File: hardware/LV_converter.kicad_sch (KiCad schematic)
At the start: 29 parts, among them IC3 AP74502QTA8-7, J9 Conn_01x02, Q11 IRLML0030, Q4 NVMFWS1D7N04XMT1G, Q5 NVMFWS1D7N04XMT1G, U8 INA228

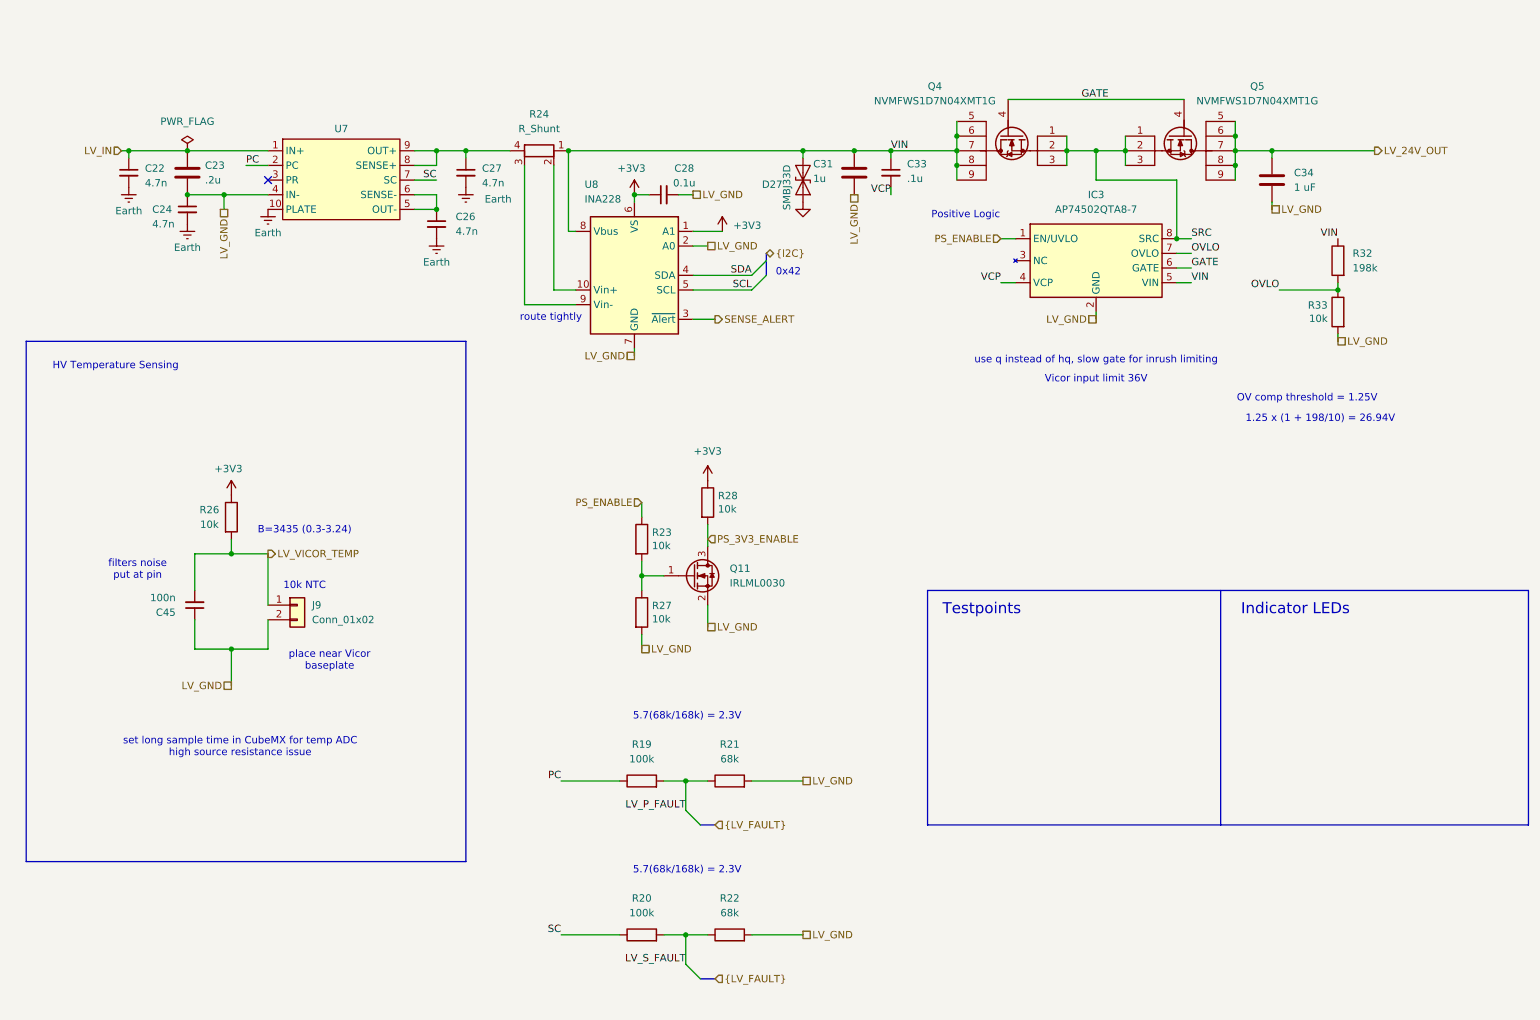
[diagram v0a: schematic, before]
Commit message: more fix, clean up, add some debug led and testpoints
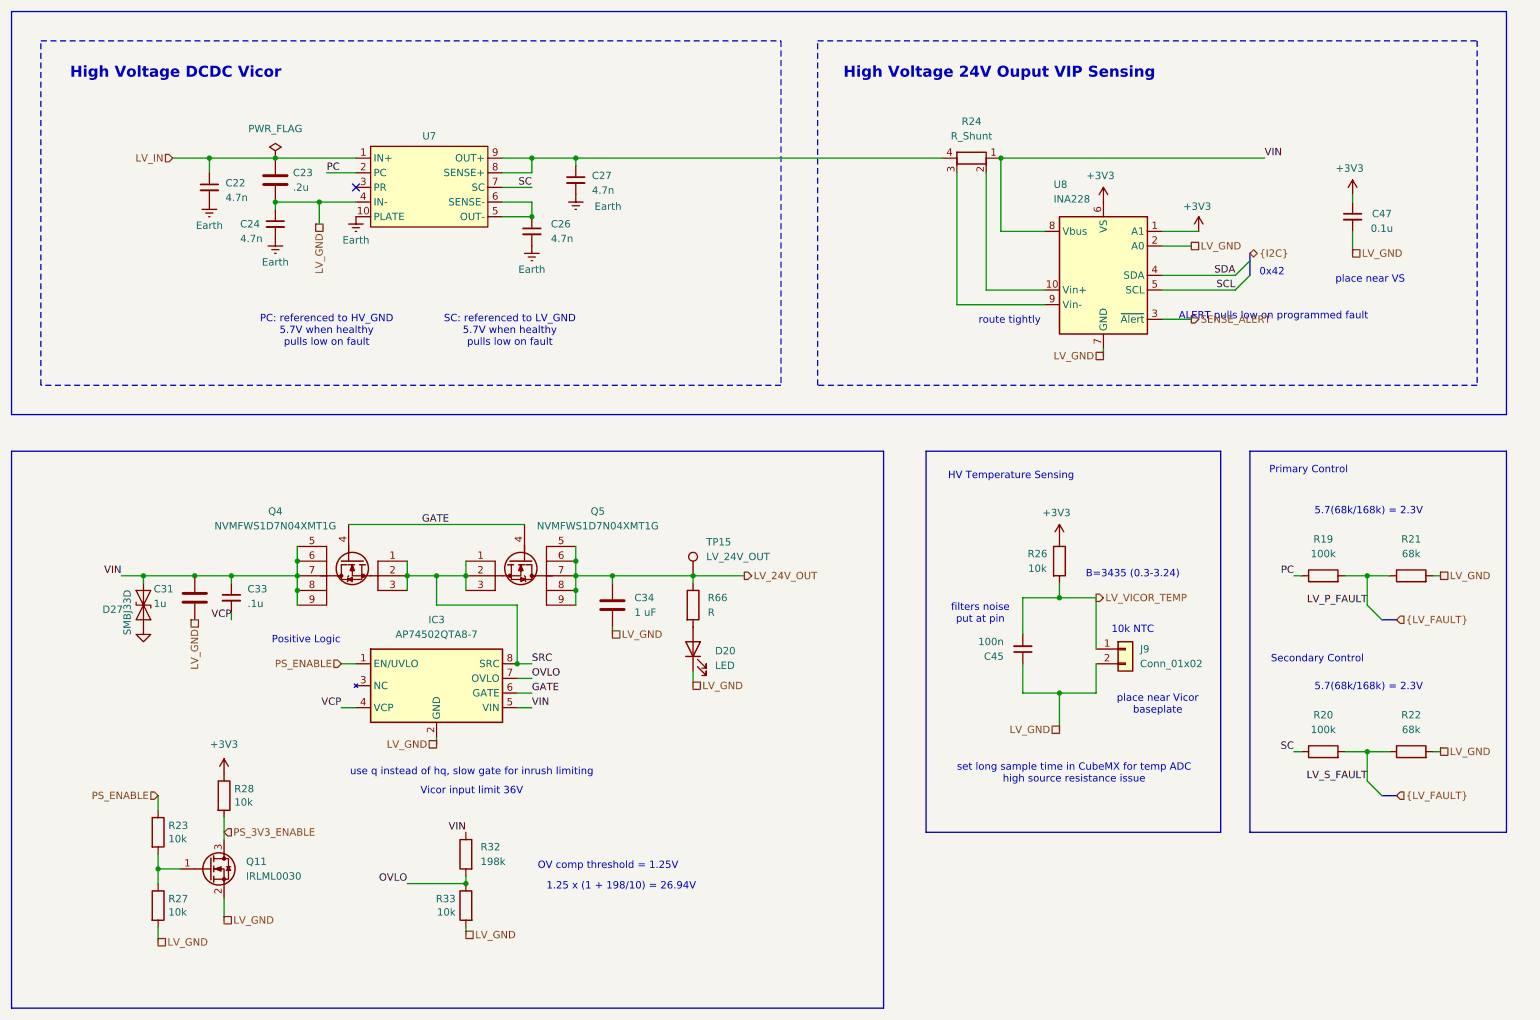
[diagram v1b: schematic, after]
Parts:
- removed C28: 0.1u, symbol Device:C_Small
- added C47: 0.1u, symbol Device:C_Small
- added D20: LED, symbol Device:LED
- added R66: R, symbol Device:R
- added TP15: LV_24V_OUT, symbol Connector:TestPoint
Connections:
- net +3V3: now also C47.1
- net LV_24V_OUT: now also R66.1, TP15.1
- net LV_GND: now also C47.2, D20.1 (K)
- new net: D20.2 (A), R66.2
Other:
- note added: "ALERT pulls low on programmed fault"
- note added: "High Voltage 24V Ouput VIP Sensing"
- note added: "High Voltage DCDC Vicor"
- note added: "PC: referenced to HV_GND 5.7V when healthy pulls low on fault"
- note added: "Primary Control"
- note added: "SC: referenced to LV_GND 5.7V when healthy pulls low on fault"
- note added: "Secondary Control"
- note added: "place near VS"
- note removed: "Indicator LEDs"
- note removed: "Testpoints"
- moved on the sheet: C22, C23, C24, C26, C27, C31, C33, C34, C45, D27, IC3, J9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
